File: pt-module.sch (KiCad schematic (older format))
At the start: 6 parts

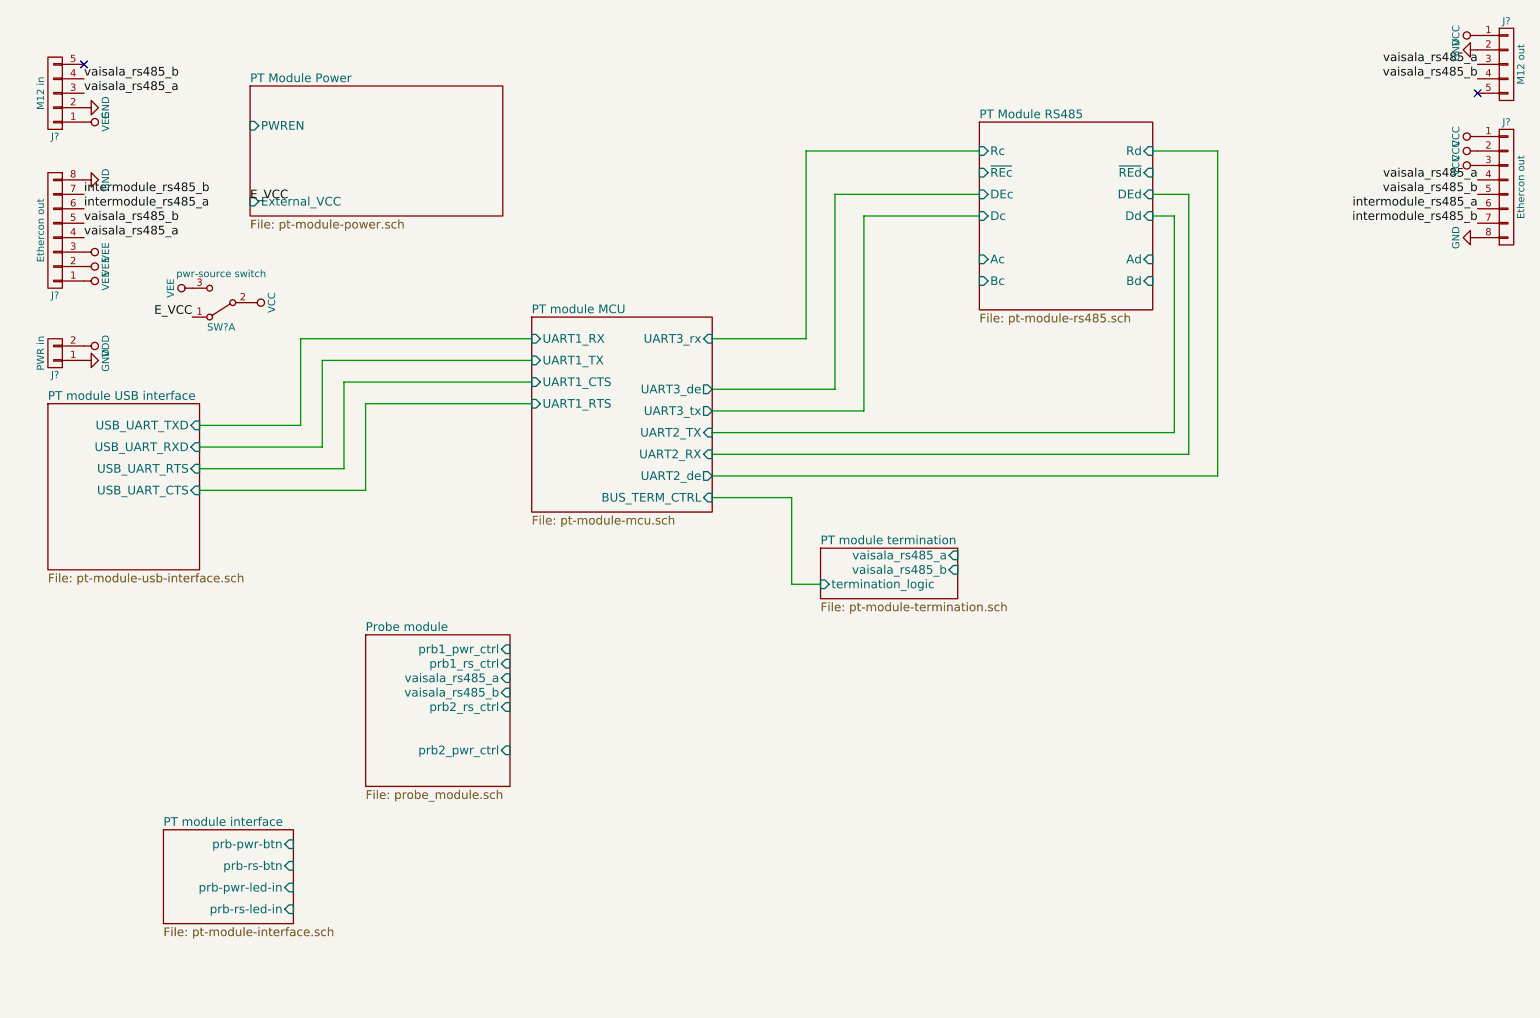
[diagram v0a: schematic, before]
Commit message: I made a connect
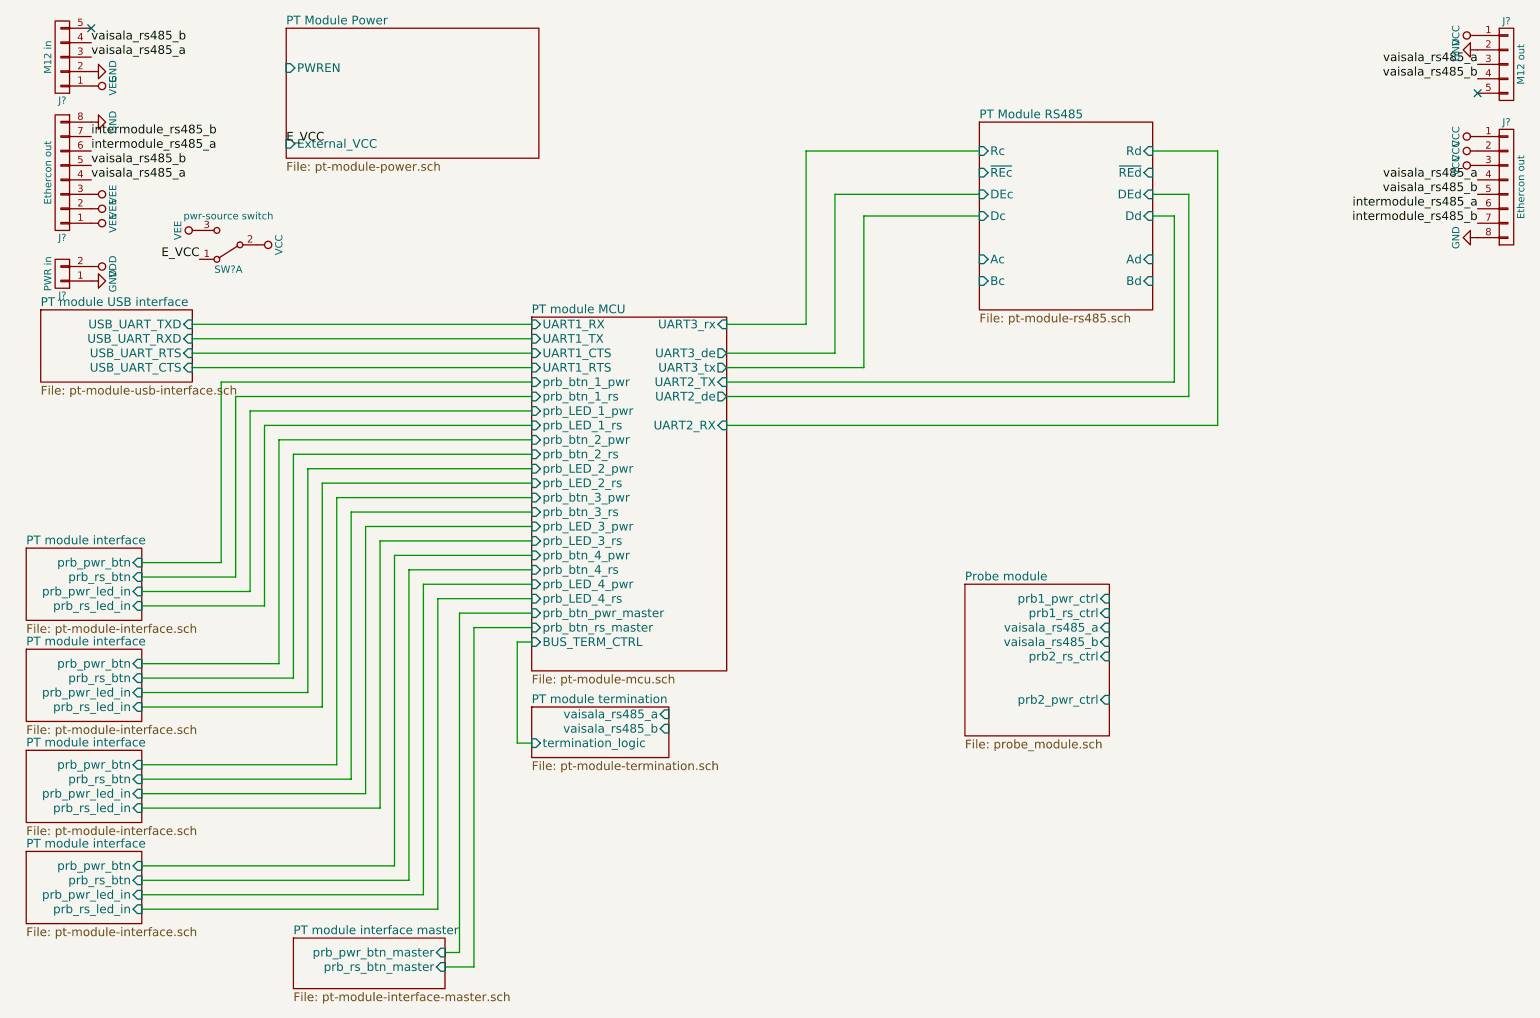
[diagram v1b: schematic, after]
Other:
- moved on the sheet: J?, SW?A
